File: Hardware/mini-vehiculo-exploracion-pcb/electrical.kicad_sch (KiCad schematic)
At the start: 21 parts, among them IC2 TPS564257DRLR

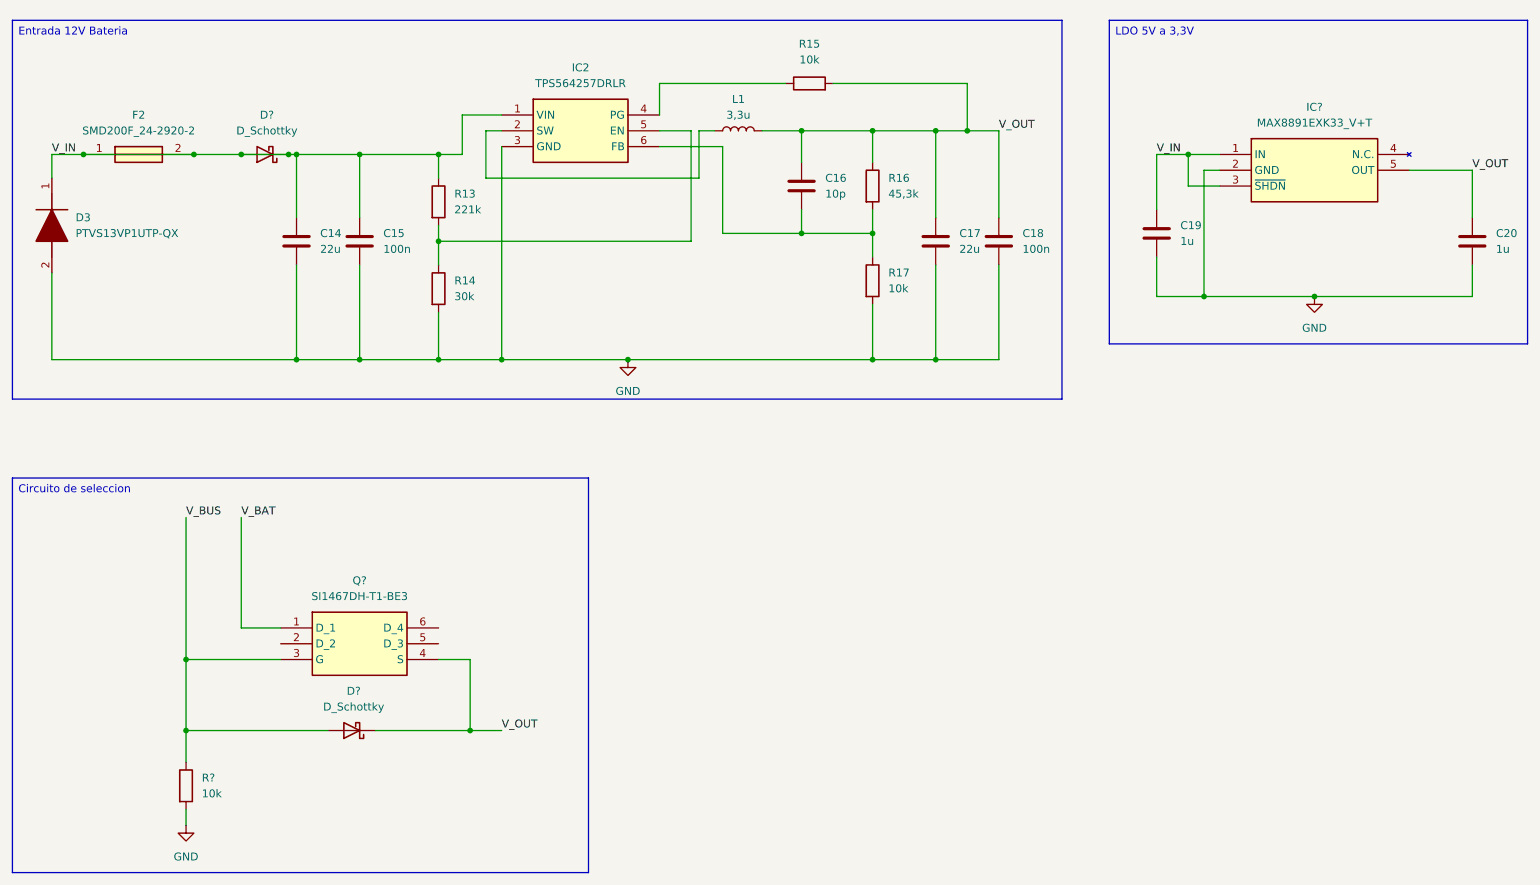
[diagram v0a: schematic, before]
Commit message: cambios
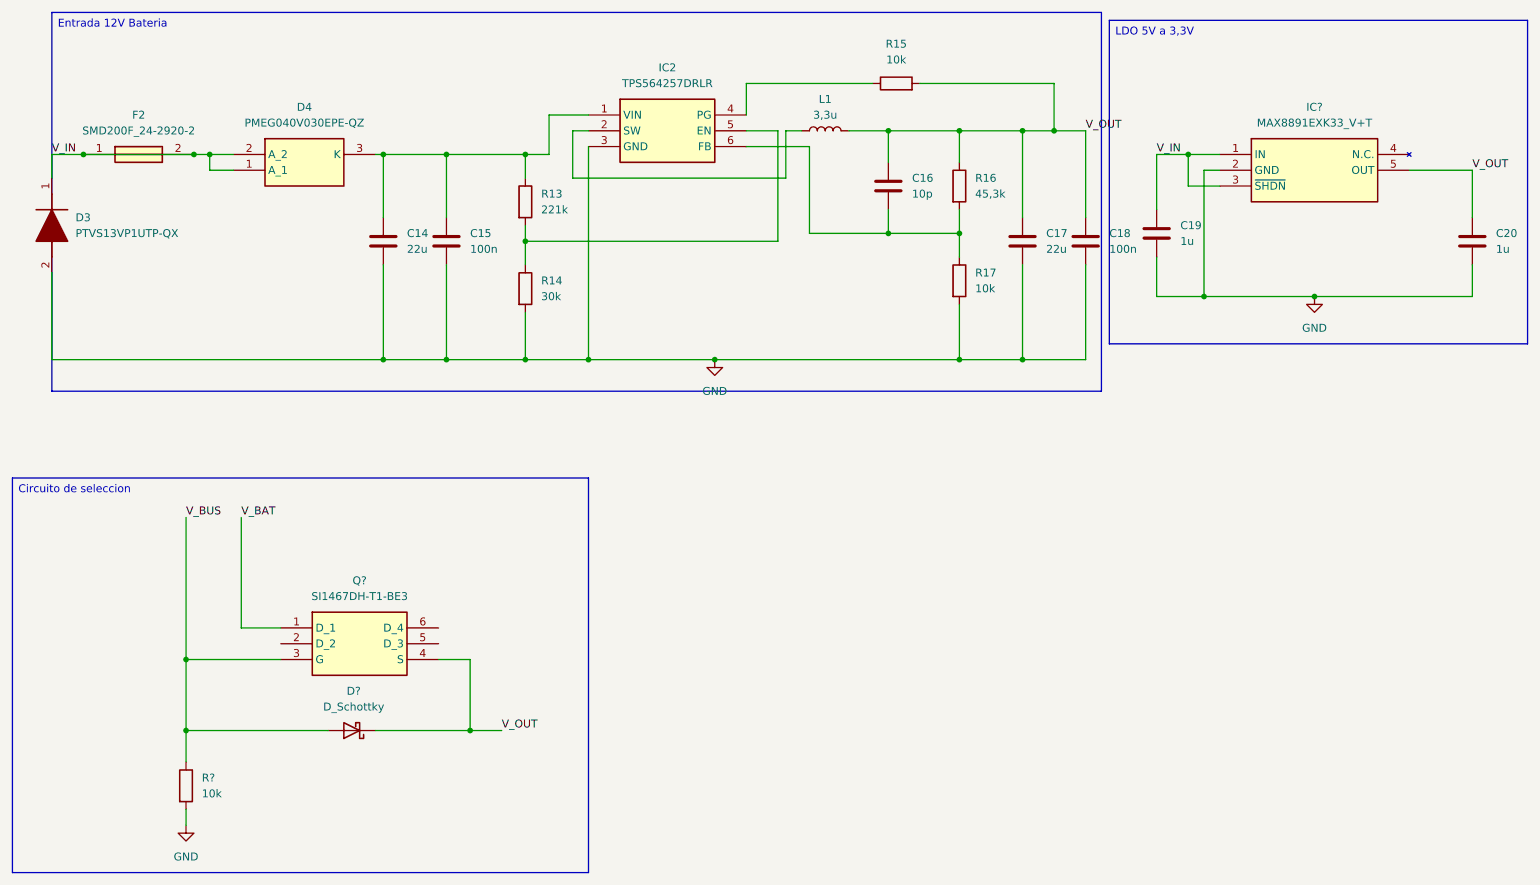
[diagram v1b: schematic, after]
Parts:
- removed D?: D_Schottky, symbol Device:D_Schottky
- added D4: PMEG040V030EPE-QZ, PMEG040V030EPEQZ, symbol PMEG040V030EPE-QZ:PMEG040V030EPE-QZ
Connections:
- net V_IN: now also D4.1 (A_1), D4.2 (A_2); no longer C14.1, C15.1, IC2.1 (VIN), R13.1
- new net: C14.1, C15.1, D4.3 (K), IC2.1 (VIN), R13.1
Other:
- moved on the sheet: C14, C15, C16, C17, C18, IC2, L1, R13, R14, R15, R16, R17
